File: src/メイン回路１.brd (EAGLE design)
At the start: 20 parts

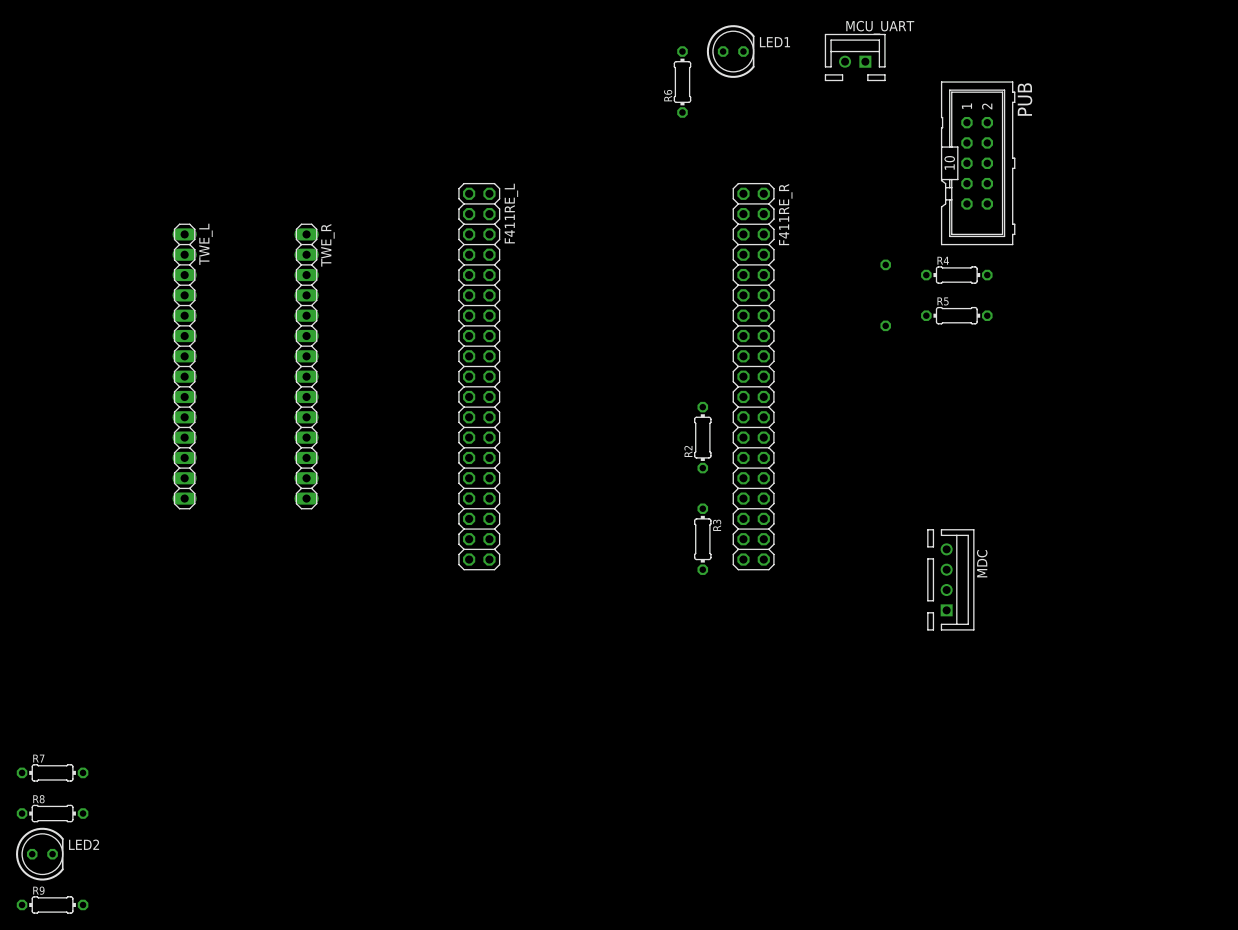
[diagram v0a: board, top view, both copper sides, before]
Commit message: [complete]メイン回路1の完成
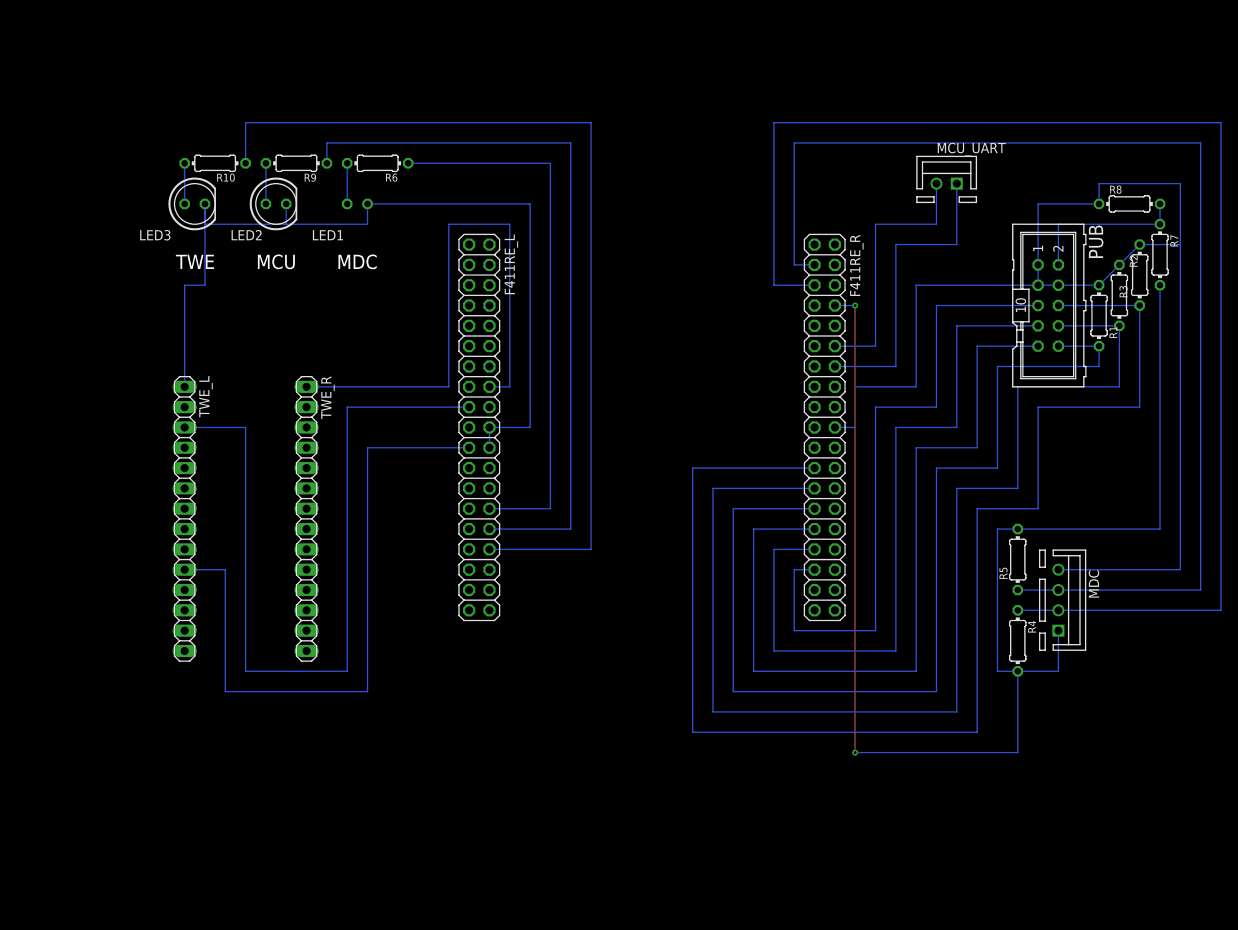
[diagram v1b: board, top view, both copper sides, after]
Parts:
- removed U$3: (no value), prototyping-board (2):TYPE.B
- added LED3: (no value), led:LED5MM
- added R10: 100, rcl:0204/7
- added U$1: (no value), prototyping-board:TYPE.B
- U$2: device prototyping-board (2):TYPE.B -> prototyping-board:TYPE.B
- moved R8 154.7 mm to (118.1, 58.4)
- moved R7 152.8 mm to (121.9, 52.1), turned to 270 degrees
- moved U$2 152.5 mm to (132.1, -15.2), flipped to the top
- moved R9 97.6 mm to (14.0, 63.5), turned to 180 degrees
- moved LED2 86.4 mm to (11.4, 58.4)
- moved R3 63.8 mm to (119.4, 49.5)
- moved R2 55.0 mm to (116.8, 47.0), turned to 270 degrees
- moved LED1 50.7 mm to (21.6, 58.4), flipped to the bottom, turned to 180 degrees
- moved R4 46.4 mm to (104.1, 3.81), turned to 270 degrees
- moved R6 39.4 mm to (24.1, 63.5), turned to 180 degrees
- moved R5 31.4 mm to (104.1, 14.0), turned to 90 degrees
- moved R1 26.8 mm to (114.3, 44.5), flipped to the top
- moved PUB 19.9 mm to (108.0, 45.7)
- moved MCU_UART 19.1 mm to (95.2, 61.0)
- moved TWE_L 19.1 mm to (0.00, 19.1)
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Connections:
- new net LED3: F411RE_L.32, R10.1
- new net N$3: LED3.A, R10.2
- net DIR1: now also F411RE_R.29; no longer F411RE_R.27
- net DIR2: now also F411RE_R.31; no longer F411RE_R.25
- net DIR3: now also F411RE_R.33; no longer F411RE_R.23
- net GND: now also LED3.K, PUB.3, PUB.4
- net LED1: now also F411RE_L.28; no longer F411RE_R.11
- net LED2: now also F411RE_L.30; no longer F411RE_R.21
- net PWM1: now also F411RE_R.27; no longer F411RE_R.29
- net PWM2: now also F411RE_R.25; no longer F411RE_R.31
- net PWM3: now also F411RE_R.23; no longer F411RE_R.33
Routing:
- net GND: track 0.00 -> 266.3 mm
- net U5V: track 0.00 -> 170.2 mm, vias 0 -> 2
- net SDA: track 0.00 -> 167.6 mm
- net PWM3: track 0.00 -> 167.6 mm
- net SCL: track 0.00 -> 147.3 mm
- net PWM2: track 0.00 -> 147.3 mm
- net PWM1: track 0.00 -> 127.0 mm
- net LED3: track 0.00 -> 114.3 mm
- net DIR1: track 0.00 -> 101.6 mm
- net RX: track 0.00 -> 99.1 mm
- net DIR2: track 0.00 -> 91.4 mm
- net LED2: track 0.00 -> 91.4 mm
- net TX: track 0.00 -> 81.3 mm
- net DIR3: track 0.00 -> 81.3 mm
- net LED1: track 0.00 -> 68.6 mm
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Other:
- board text added: "MCU"
- board text added: "MDC"
- board text added: "TWE"
